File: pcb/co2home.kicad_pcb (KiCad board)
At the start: 2 copper layers, 40.6 x 75.8 mm, 11 parts, among them J1 esp32buddy, J2 USB_B_Micro, U1 MH-Z19, U2 TLV75533PDBV, U3 ESP32-WROOM-32D

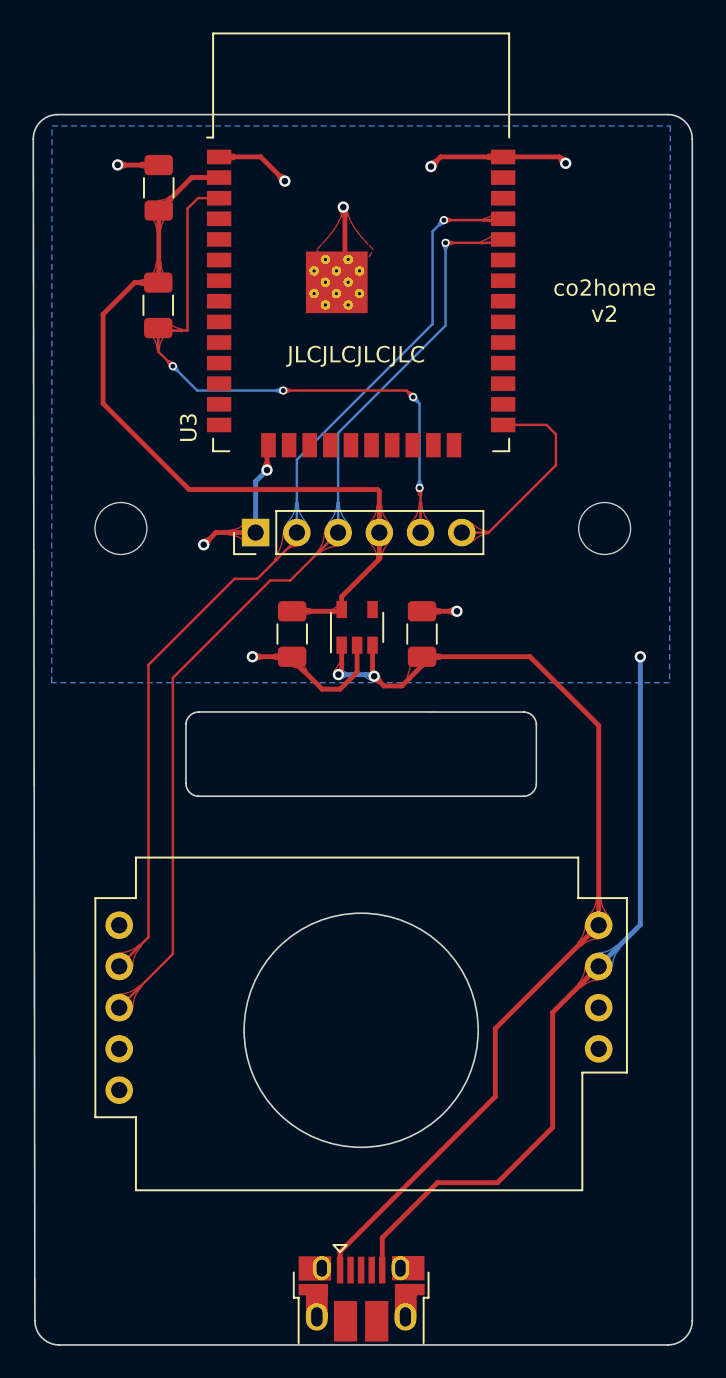
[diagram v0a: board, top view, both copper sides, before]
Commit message: newness
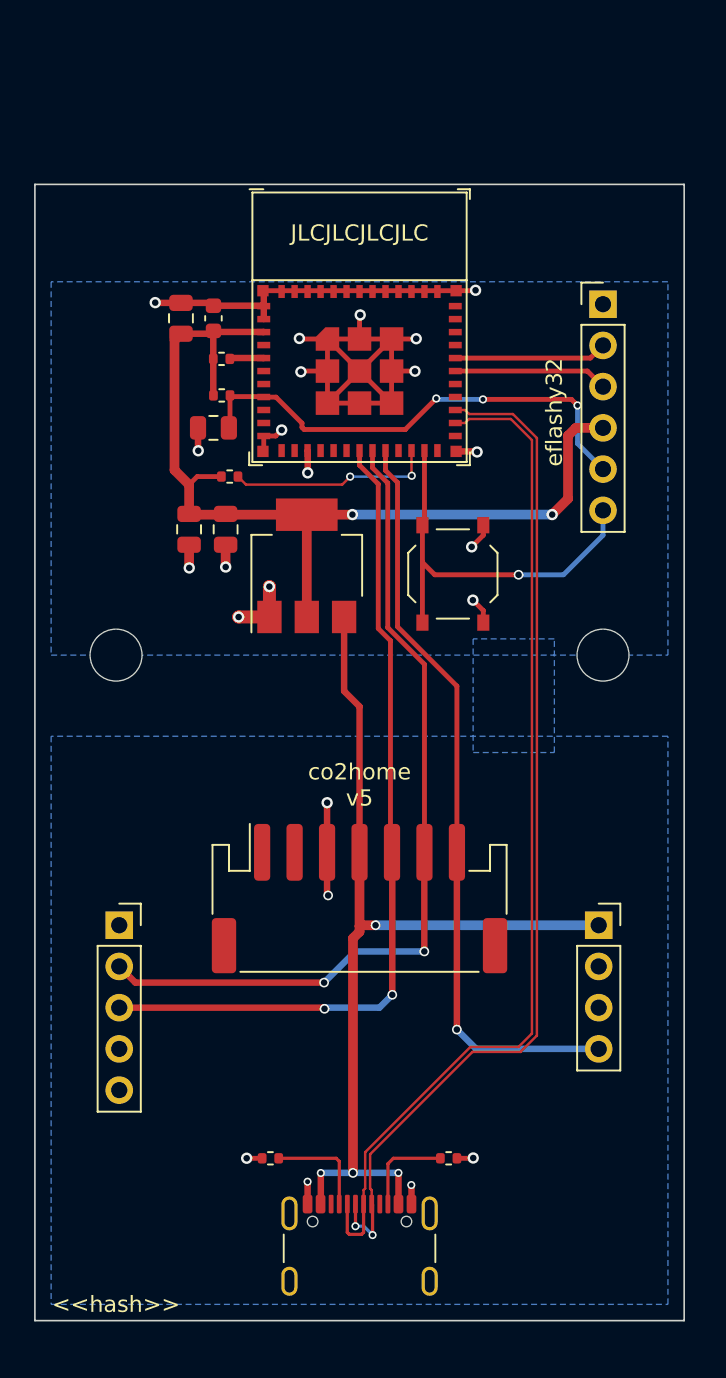
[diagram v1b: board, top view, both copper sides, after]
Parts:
- removed C1, C2: 1uF, Capacitor_SMD:C_1206_3216Metric
- removed C3: 10uF, Capacitor_SMD:C_1206_3216Metric
- removed R1: 100k, Resistor_SMD:R_1206_3216Metric
- removed REF** (x2): MountingHole_3.2mm_M3, MountingHole:MountingHole_3.2mm_M3
- removed U2: TLV75533PDBV, Package_TO_SOT_SMD:SOT-23-5
- removed U3: ESP32-WROOM-32D, RF_Module:ESP32-WROOM-32D
- added C4: 10u, Capacitor_SMD:C_0805_2012Metric, F.Cu at (125.9, 49.7)
- added C5: 0.1u, Capacitor_SMD:C_0603_1608Metric, F.Cu at (125.9, 43.0)
- added C6: 10u, Capacitor_SMD:C_0805_2012Metric, F.Cu at (123.9, 43.0)
- added C7: 10u, Capacitor_SMD:C_0805_2012Metric, F.Cu at (126.7, 56.0)
- added C8: 10u, Capacitor_SMD:C_0805_2012Metric, F.Cu at (124.4, 56.0)
- added H1: MountingHole, MountingHole:MountingHole_3.2mm_M3, F.Cu at (119.9, 63.7)
- added H2: MountingHole, MountingHole:MountingHole_3.2mm_M3, F.Cu at (149.9, 63.7)
- added J3: USBC, Connector_USB:USB_C_Receptacle_GCT_USB4105-xx-A_16P_TopMnt_Horizontal, F.Cu at (134.9, 101.2)
- added J4: MH-Z19 R, Connector_PinSocket_2.54mm:PinSocket_1x04_P2.54mm_Vertical, F.Cu at (149.7, 80.3)
- added J5: JST-PH, Connector_JST:JST_PH_S7B-PH-SM4-TB_1x07-1MP_P2.00mm_Horizontal, F.Cu at (134.9, 78.7)
- added R2: 5k1, Resistor_SMD:R_0402_1005Metric, F.Cu at (140.4, 94.7)
- added R3: 5k1, Resistor_SMD:R_0402_1005Metric, F.Cu at (129.4, 94.7)
- added R4: 10k, Resistor_SMD:R_0402_1005Metric, F.Cu at (126.4, 47.7)
- added R5: 10k, Resistor_SMD:R_0402_1005Metric, F.Cu at (126.4, 45.5)
- added R6: 10k, Resistor_SMD:R_0402_1005Metric, F.Cu at (126.9, 52.7)
- added SW1: RESET, Button_Switch_SMD:SW_Push_1P1T_XKB_TS-1187A, F.Cu at (140.7, 58.7)
- added U4: AMS1117-3.3, Package_TO_SOT_SMD:SOT-223-3_TabPin2, F.Cu at (131.7, 58.2)
- J1: value esp32buddy -> eflashy32
- J2: value USB_B_Micro -> MH-Z19 L; footprint !Greg:USB_Micro-B_Amphenol_10103594-0001LF_Horizontal -> Connector_PinSocket_2.54mm:PinSocket_1x05_P2.54mm_Vertical
- U1: value MH-Z19 -> ESP32-C3-MINI-1; footprint !Greg:MH-Z19 -> Espressif:ESP32-C3-MINI-1
- moved U1 42.0 mm to (134.9, 43.5), turned to 0 degrees
- moved J2 27.4 mm to (120.1, 80.3)
- moved J1 25.6 mm to (149.9, 42.1), turned to 0 degrees
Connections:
- J1 pad 2: /TXD -> /PROGTXD
- J1 pad 3: /RXD -> /PROGRXD
- J2 pad 1: VBUS -> unconnected-(J2-Pin_1-Pad1)
- J2 pad 2: (no net) -> TXD
- J2 pad 3: (no net) -> RXD
- J2 pad 4: (no net) -> unconnected-(J2-Pin_4-Pad4)
- J2 pad 5: GND -> unconnected-(J2-Pin_5-Pad5)
- U1 pad 1: (no net) -> GND
- U1 pad 2: /TXD -> GND
- U1 pad 3: /RXD -> +3V3
- U1 pad 4: (no net) -> unconnected-(U1-NC-Pad4)
- U1 pad 5: (no net) -> Net-(U1-GPIO2/ADC1_CH2)
- U1 pad 6: VBUS -> unconnected-(U1-GPIO3/ADC1_CH3-Pad6)
- U1 pad 7: GND -> unconnected-(U1-NC-Pad7)
- U1 pad 8: (no net) -> /EN
- U1 pad 9: (no net) -> unconnected-(U1-NC-Pad9)
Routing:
- net D+: track 0.00 -> 63.5 mm, vias 0 -> 2
- net VBUS: track 63.1 -> 0.00 mm, vias 2 -> 0
- net D-: track 0.00 -> 63.1 mm
- net /RXD: track 59.6 -> 0.00 mm, vias 1 -> 0
- net /TXD: track 58.5 -> 0.00 mm, vias 1 -> 0
- net +5V: track 0.00 -> 58.2 mm, vias 0 -> 4
- net TXD: track 0.00 -> 52.2 mm, vias 0 -> 2
- net RXD: track 0.00 -> 51.6 mm, vias 0 -> 2
- net PWM: track 0.00 -> 46.7 mm, vias 0 -> 1
- net Net-(U1-GPIO8): track 0.00 -> 12.7 mm, vias 0 -> 2
- net /GPIO0: track 13.2 -> 24.6 mm, vias 0 -> 1
- net +3V3: track 49.8 -> 59.3 mm, vias 0 -> 2
- net /PROGRXD: track 0.00 -> 9.50 mm
- net /PROGTXD: track 0.00 -> 9.42 mm
- net /EN: track 38.7 -> 30.0 mm, vias 4 -> 3
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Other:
- board size 40.6 x 75.8 mm -> 40 x 70 mm
- board text added: "<<hash>>"
- board text added: "Thermal break"
- board text added: "co2home v5"
- board text removed: "co2home v2"
